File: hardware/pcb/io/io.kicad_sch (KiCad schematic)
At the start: 14 parts, among them J1 Conn_02x08_Odd_Even, J2 DIN-3, J3 DIN-3, J4 DIN-3, J5 DIN-3, J6 Conn_01x04

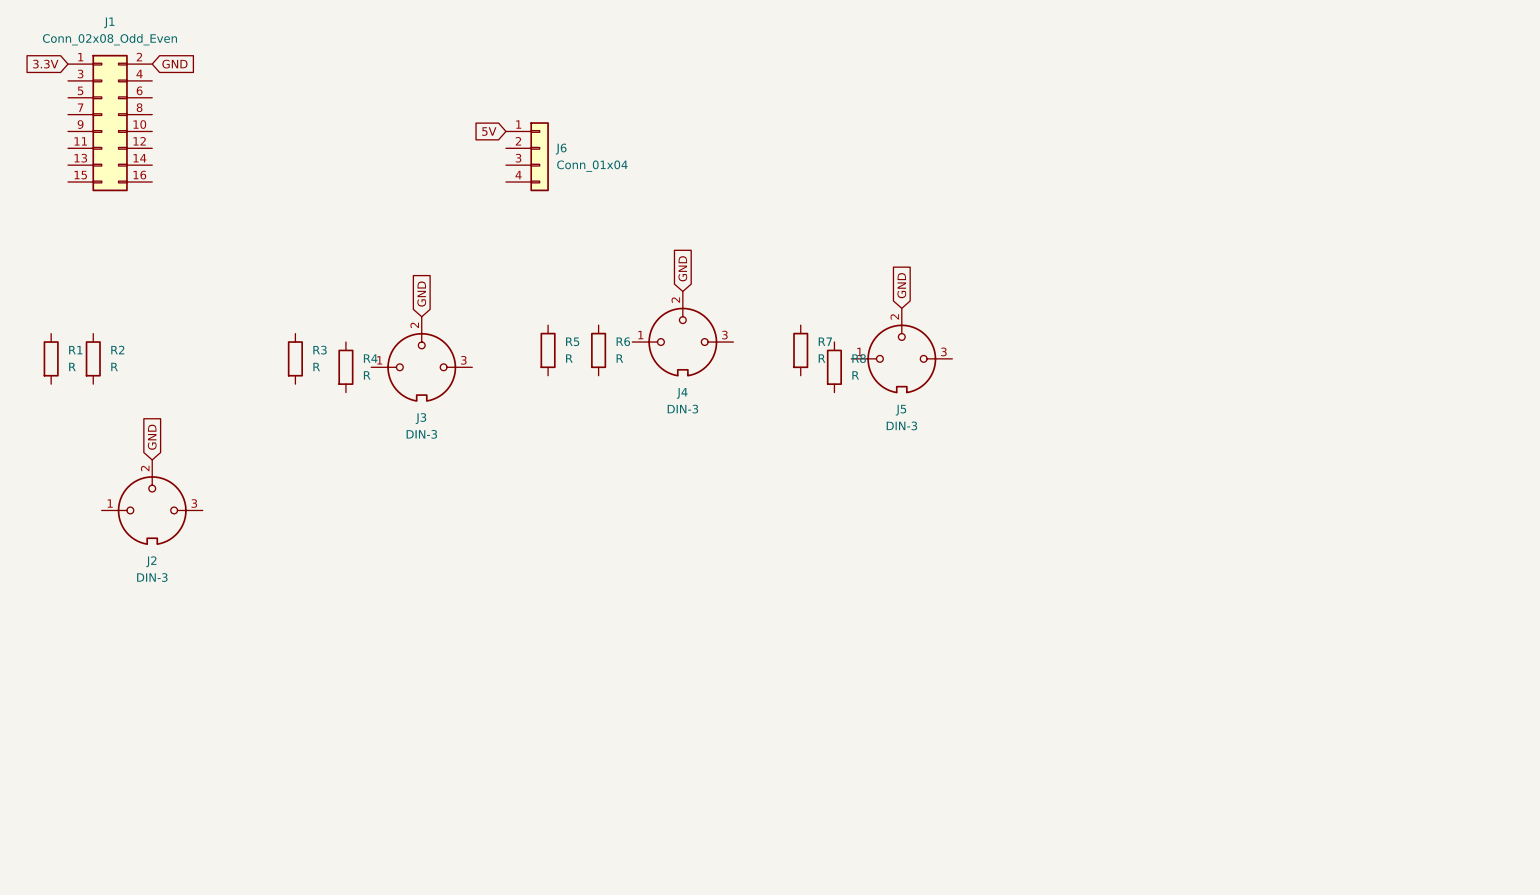
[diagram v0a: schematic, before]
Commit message: pcb: version 1 for all boards
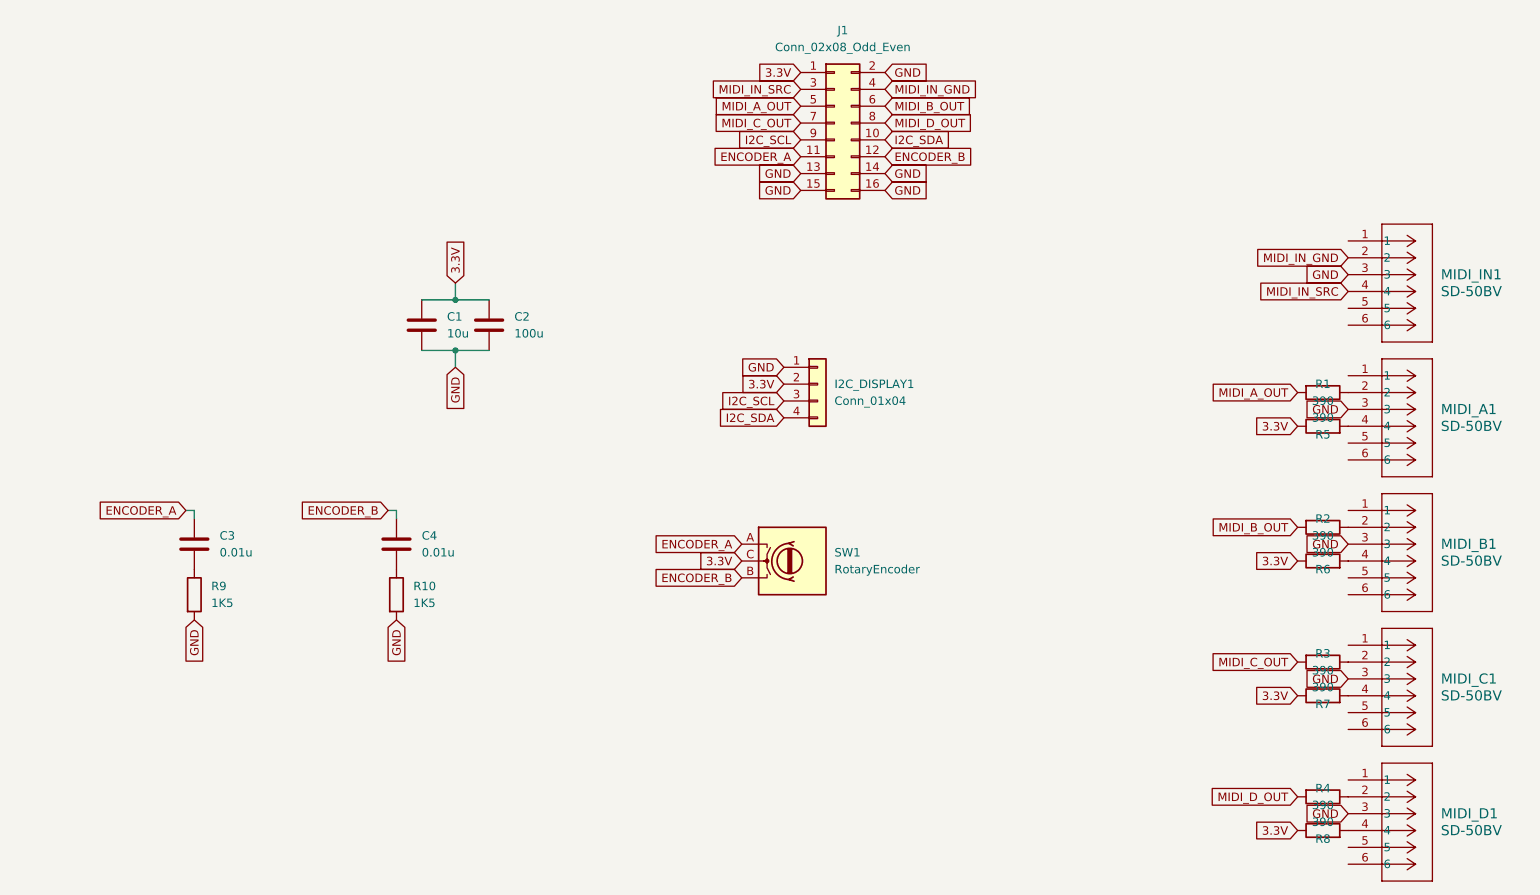
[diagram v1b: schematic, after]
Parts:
- removed J2, J3, J4, J5: DIN-3, symbol Connector:DIN-3
- added C1: 10u, Capacitor_THT:CP_Radial_D5.0mm_P2.50mm, symbol Device:C
- added C2: 100u, Capacitor_THT:CP_Radial_D5.0mm_P2.50mm, symbol Device:C
- added C3, C4: 0.01u, Capacitor_THT:CP_Radial_D5.0mm_P2.50mm, symbol Device:C
- added MIDI_A1, MIDI_B1, MIDI_C1, MIDI_D1, MIDI_IN1: SD-50BV, footprints:CONN6_SD-50BV_CUD, symbol 2025-04-25_22-15-08:SD-50BV
- added R10, R9: 1K5, Resistor_THT:R_Axial_DIN0207_L6.3mm_D2.5mm_P10.16mm_Horizontal, symbol Device:R
- added SW1: RotaryEncoder, rotary-encoder-PEC11R-main:Bourns-PEC11R-4220F-S0024-0-0-0, symbol Device:RotaryEncoder
- I2C_DISPLAY1: renamed from J6; footprint (none) -> Connector_PinHeader_2.54mm:PinHeader_1x04_P2.54mm_Vertical
- J1: footprint (none) -> Connector_PinHeader_2.54mm:PinHeader_2x08_P2.54mm_Vertical
- R1, R2, R3, R4, R5, R6, R7, R8: value R -> 390; footprint (none) -> Resistor_THT:R_Axial_DIN0207_L6.3mm_D2.5mm_P10.16mm_Horizontal
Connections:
- net 5V is gone; now on net GND: I2C_DISPLAY1.1 (Pin_1)
- net 3.3V: now also I2C_DISPLAY1.2 (Pin_2), R1.1, R2.1, R3.1, R4.1, C1.1, C2.1, SW1.C
- net GND: now also J1.13 (Pin_13), J1.14 (Pin_14), J1.15 (Pin_15), J1.16 (Pin_16), C1.2, C2.2, MIDI_A1.3, MIDI_B1.3, MIDI_C1.3, MIDI_D1.3, MIDI_IN1.3, R10.2, R9.2
- net at R8.1: now also MIDI_D1.2
- net MIDI_D_OUT: now reaches R8.2
- net MIDI_D_OUT: now also J1.8 (Pin_8)
- net at R1.2: now also MIDI_A1.4
- net at R7.1: now also MIDI_C1.2
- net MIDI_C_OUT: now reaches R7.2
- net MIDI_C_OUT: now also J1.7 (Pin_7)
- net at R6.1: now also MIDI_B1.2
- net MIDI_B_OUT: now reaches R6.2
- net MIDI_B_OUT: now also J1.6 (Pin_6)
- net at R4.2: now also MIDI_D1.4
- net I2C_SCL: now reaches I2C_DISPLAY1.3 (Pin_3)
- net I2C_SCL: now also J1.9 (Pin_9)
- net I2C_SDA: now reaches I2C_DISPLAY1.4 (Pin_4)
- net I2C_SDA: now also J1.10 (Pin_10)
- net ENCODER_A: now reaches J1.11 (Pin_11)
- net ENCODER_A: now also C3.1, SW1.A
- net ENCODER_B: now reaches J1.12 (Pin_12)
- net ENCODER_B: now also C4.1, SW1.B
- net MIDI_IN_SRC: now reaches J1.3 (Pin_3)
- net MIDI_IN_SRC: now also MIDI_IN1.4
- net MIDI_IN_GND: now reaches J1.4 (Pin_4)
- net MIDI_IN_GND: now also MIDI_IN1.2
- net MIDI_A_OUT: now reaches J1.5 (Pin_5)
- net MIDI_A_OUT: now also R5.2
- net at R3.2: now also MIDI_C1.4
- net at R5.1: now also MIDI_A1.2
- net at R2.2: now also MIDI_B1.4
- new net: C3.2, R9.1
- new net: C4.2, R10.1
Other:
- moved on the sheet: I2C_DISPLAY1, J1
